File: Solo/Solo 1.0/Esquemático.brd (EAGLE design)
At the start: 51 x 57 mm, 13 parts, among them Q1 IRF540, Q2 IRF540, Q3 IRF540

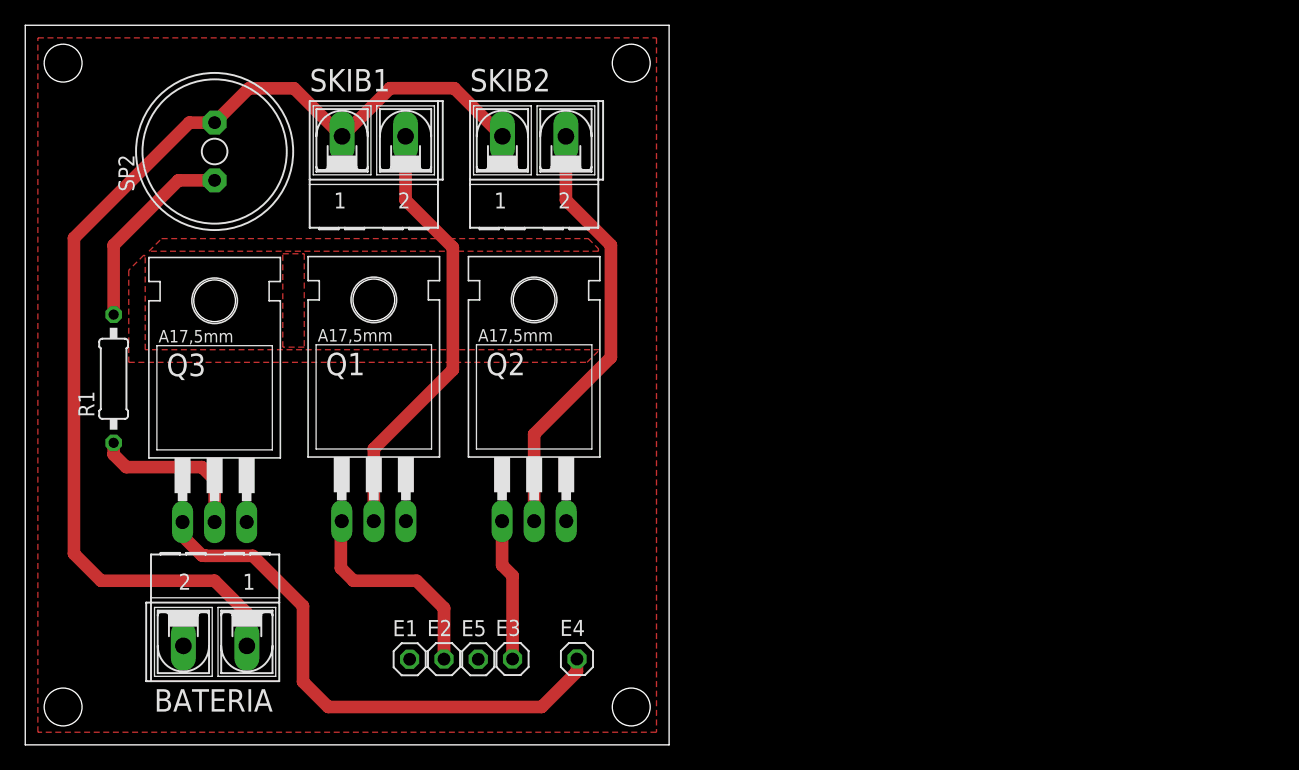
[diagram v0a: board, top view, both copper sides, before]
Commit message: Message
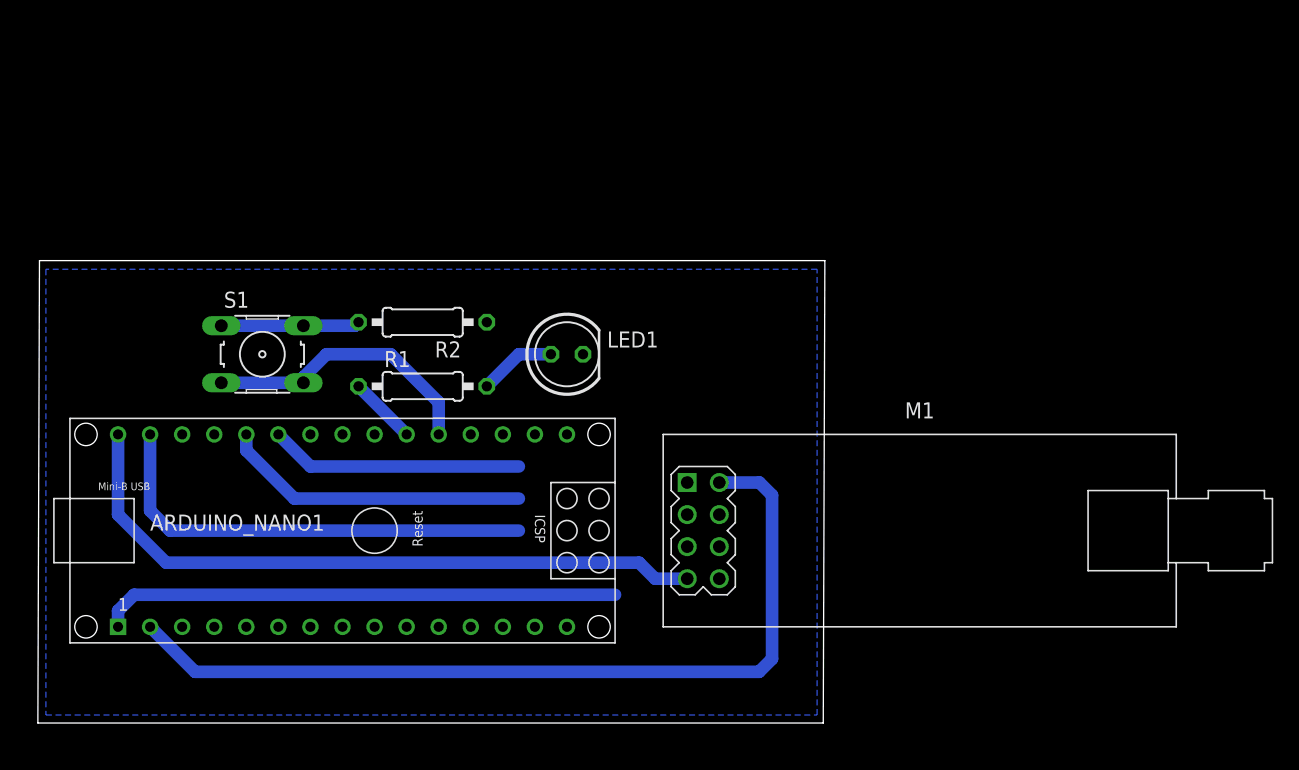
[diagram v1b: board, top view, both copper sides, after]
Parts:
- removed BATERIA, SKIB1, SKIB2: (no value), con-ptr500:AK500/2-H
- removed E1: 3V3, pinhead:1X01
- removed E2: SKIB1, pinhead:1X01
- removed E3: SKIB2, pinhead:1X01
- removed E4: BUZZER, pinhead:1X01
- removed E5: GND, pinhead:1X01
- removed Q1, Q2, Q3: IRF540, transistor-fet:TO220
- removed SP2: AL11P, buzzer:AL11P
- added ARDUINO_NANO1: (no value), ArduinoNanoV30:ARDUINO_NANO
- added LED1: (no value), led:LED5MM
- added M1: WIRELESS-NRF24L01-PA-EXT, modules:WIRELESS-NRF24L01-PA-EXT
- added R2: (no value), rcl:0207/10
- added S1: (no value), switch-omron:B3F-10XX
- R1: value 330 -> (none)
- moved R1 24.5 mm to (30.5, 25.4), turned to 0 degrees
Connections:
- removed net 3.3V: E1.1
- removed net BUZZER: E4.1, Q3.1
- removed net S1: Q1.2, SKIB1.2
- removed net S2: Q2.2, SKIB2.2
- removed net SKIB1: E2.1, Q1.1
- removed net SKIB2: E3.1, Q2.1
- removed net VCC: BATERIA.1, SKIB1.1, SKIB2.1, SP2.+
- new net 5V: ARDUINO_NANO1.12
- new net N$1: LED1.A, R1.2
- new net N$10: ARDUINO_NANO1.2, M1.2
- new net N$3: R2.2, S1.1, S1.2
- new net N$5: ARDUINO_NANO1.1, M1.5
- new net N$6: ARDUINO_NANO1.30, M1.7
- new net N$7: ARDUINO_NANO1.29, M1.6
- new net N$8: ARDUINO_NANO1.25, M1.3
- new net N$9: ARDUINO_NANO1.26, M1.4
- new net VIN: ARDUINO_NANO1.15
- net GND: now also ARDUINO_NANO1.14, ARDUINO_NANO1.19, LED1.K, M1.1, R2.1; no longer BATERIA.2, E5.1, Q1.3, Q2.3, Q3.3
- net N$2: now also ARDUINO_NANO1.20, S1.3, S1.4; no longer Q3.2, R1.1
- net N$4: now also ARDUINO_NANO1.21, R1.1; no longer R1.2, SP2.-
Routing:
- net VCC: track 86.8 -> 0.00 mm
- net N$10: track 0.00 -> 68.7 mm
- net N$6: track 0.00 -> 53.5 mm
- net BUZZER: track 43.6 -> 0.00 mm
- net N$5: track 0.00 -> 41.2 mm
- net N$7: track 0.00 -> 35.9 mm
- net S1: track 34.6 -> 0.00 mm
- net S2: track 34.5 -> 0.00 mm
- net N$9: track 0.00 -> 24.4 mm
- net N$8: track 0.00 -> 20.1 mm
- net SKIB1: track 17.3 -> 0.00 mm
- net SKIB2: track 11.3 -> 0.00 mm
- net N$3: track 0.00 -> 11.0 mm
- net N$4: track 15.6 -> 5.39 mm
- net N$2: track 13.1 -> 22.7 mm
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- added copper zone on layer 16, net GND
- removed copper zone on layer 1, net DS
- removed copper zone on layer 1, net GND
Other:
- board size 51 x 57 mm -> 62.3 x 36.6 mm

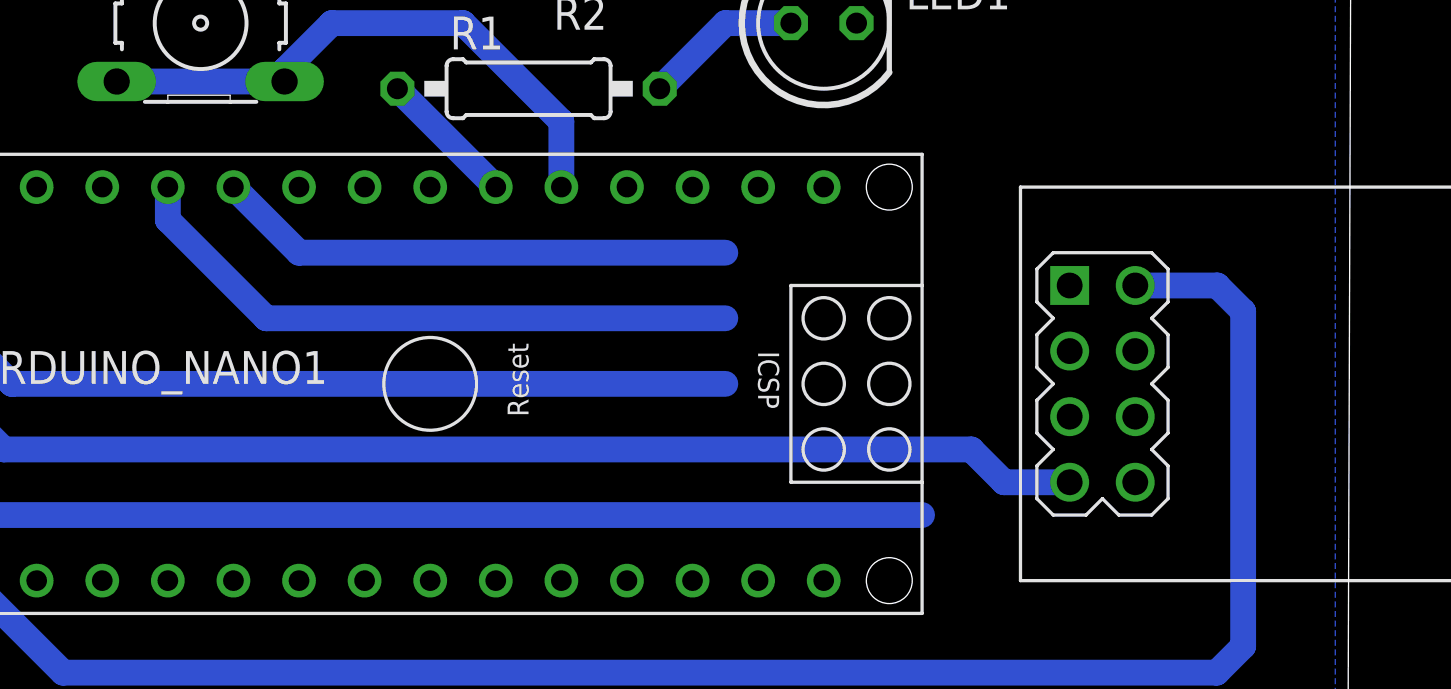
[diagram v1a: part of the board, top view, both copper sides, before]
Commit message: Upgrage
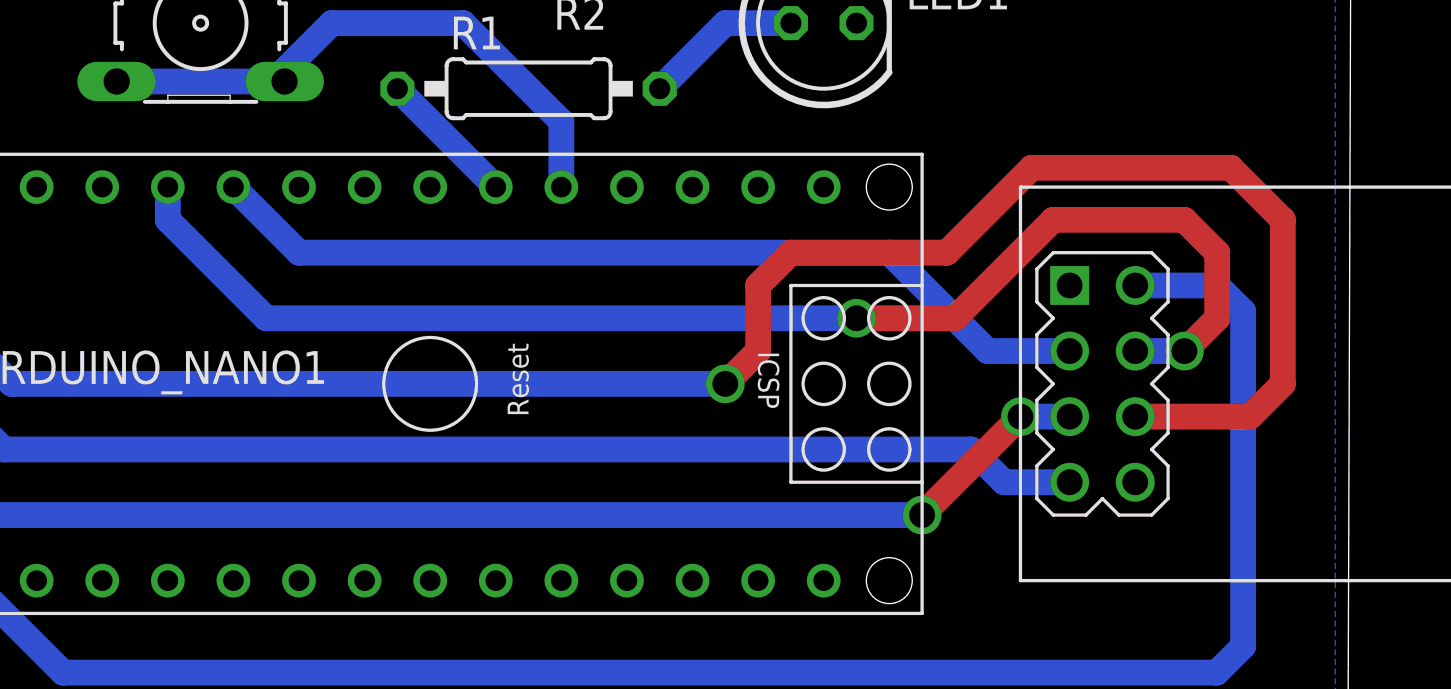
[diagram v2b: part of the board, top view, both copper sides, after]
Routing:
- net N$7: track 35.9 -> 75.9 mm, vias 0 -> 1
- net N$9: track 24.4 -> 51.8 mm, vias 0 -> 2
- net N$8: track 20.1 -> 35.0 mm
- net N$5: track 41.2 -> 48.5 mm, vias 0 -> 2
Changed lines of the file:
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@@
 <wire x1="6.35" y1="6.35" x2="6.35" y2="7.62" width="1" layer="16"/>
 <wire x1="6.35" y1="7.62" x2="7.62" y2="8.89" width="1" layer="16"/>
+<via x="45.72" y="8.89" extent="1-16" drill="1"/>
+<wire x1="49.53" y1="12.7" x2="45.72" y2="8.89" width="1" layer="1"/>
+<via x="49.53" y="12.7" extent="1-16" drill="1"/>
+<wire x1="49.53" y1="12.7" x2="51.435" y2="12.7" width="1" layer="16"/>
 <wire x1="7.62" y1="8.89" x2="45.72" y2="8.89" width="1" layer="16"/>
-<wire x1="45.72" y1="8.89" x2="51.435" y2="12.7" width="0" layer="19" extent="16-16"/>
 </signal>
 <signal name="N$6">
@@
 <wire x1="8.89" y1="15.55105625" x2="10.47105625" y2="13.97" width="1" layer="16"/>
 <wire x1="10.47105625" y1="13.97" x2="38.1" y2="13.97" width="1" layer="16"/>
-<wire x1="38.1" y1="13.97" x2="53.975" y2="12.7" width="0" layer="19" extent="16-16"/>
+<via x="38.1" y="13.97" extent="1-16" drill="1"/>
+<wire x1="38.1" y1="13.97" x2="39.37" y2="15.24" width="1" layer="1"/>
+<wire x1="39.37" y1="17.78" x2="40.64" y2="19.05" width="1" layer="1"/>
+<wire x1="40.64" y1="19.05" x2="46.67894375" y2="19.05" width="1" layer="1"/>
+<wire x1="57.674" y1="22.336" x2="59.69" y2="20.32" width="1" layer="1"/>
+<wire x1="59.69" y1="20.32" x2="59.69" y2="13.97" width="1" layer="1"/>
+<wire x1="59.69" y1="13.97" x2="58.42" y2="12.7" width="1" layer="1"/>
+<wire x1="58.42" y1="12.7" x2="53.975" y2="12.7" width="1" layer="1"/>
+<wire x1="39.37" y1="15.24" x2="39.37" y2="17.78" width="1" layer="1"/>
+<wire x1="46.67894375" y1="19.05" x2="49.96494375" y2="22.336" width="1" layer="1"/>
+<wire x1="49.96494375" y1="22.336" x2="57.674" y2="22.336" width="1" layer="1"/>
 </signal>
 <signal name="N$8">
@@
 <contactref element="ARDUINO_NANO1" pad="25"/>
 <wire x1="19.05" y1="21.59" x2="21.59" y2="19.05" width="1" layer="16"/>
-<wire x1="21.59" y1="19.05" x2="38.1" y2="19.05" width="1" layer="16"/>
-<wire x1="38.1" y1="19.05" x2="51.435" y2="15.24" width="0" layer="19" extent="16-16"/>
+<wire x1="44.45" y1="19.05" x2="48.26" y2="15.24" width="1" layer="16"/>
+<wire x1="48.26" y1="15.24" x2="51.435" y2="15.24" width="1" layer="16"/>
+<wire x1="21.59" y1="19.05" x2="44.45" y2="19.05" width="1" layer="16"/>
 </signal>
 <signal name="N$9">
 <contactref element="ARDUINO_NANO1" pad="26"/>
 <contactref element="M1" pad="4"/>
-<wire x1="20.32" y1="16.51" x2="16.51" y2="20.32" width="1" layer="16"/>
+<wire x1="16.51" y1="20.32" x2="20.32" y2="16.51" width="1" layer="16"/>
 <wire x1="16.51" y1="21.59" x2="16.51" y2="20.32" width="1" layer="16"/>
-<wire x1="20.32" y1="16.51" x2="38.1" y2="16.51" width="1" layer="16"/>
-<wire x1="38.1" y1="16.51" x2="53.975" y2="15.24" width="0" layer="19" extent="16-16"/>
+<via x="43.18" y="16.51" extent="1-16" drill="1"/>
+<wire x1="50.8" y1="20.32" x2="46.99" y2="16.51" width="1" layer="1"/>
+<wire x1="43.18" y1="16.51" x2="46.99" y2="16.51" width="1" layer="1"/>
+<wire x1="57.15" y1="19.05" x2="57.15" y2="16.51" width="1" layer="1"/>
+<via x="55.88" y="15.24" extent="1-16" drill="1"/>
+<wire x1="55.88" y1="15.24" x2="53.975" y2="15.24" width="1" layer="16"/>
+<wire x1="20.32" y1="16.51" x2="43.18" y2="16.51" width="1" layer="16"/>
+<wire x1="50.8" y1="20.32" x2="55.88" y2="20.32" width="1" layer="1"/>
+<wire x1="55.88" y1="20.32" x2="57.15" y2="19.05" width="1" layer="1"/>
+<wire x1="57.15" y1="16.51" x2="55.88" y2="15.24" width="1" layer="1"/>
 </signal>
 <signal name="N$10">
-<contactref element="M1" pad="2"/>
 <contactref element="ARDUINO_NANO1" pad="2"/>
 <wire x1="8.89" y1="6.35" x2="12.454" y2="2.786" width="1" layer="16"/>
 <wire x1="57.13" y1="2.786" x2="58.154" y2="3.81" width="1" layer="16"/>
 <wire x1="58.154" y1="16.776" x2="57.15" y2="17.78" width="1" layer="16"/>
-<wire x1="57.15" y1="17.78" x2="53.975" y2="17.78" width="1" layer="16"/>
 <wire x1="12.454" y1="2.786" x2="57.13" y2="2.786" width="1" layer="16"/>
 <wire x1="58.154" y1="3.81" x2="58.154" y2="16.776" width="1" layer="16"/>
+<contactref element="M1" pad="2"/>
+<wire x1="57.15" y1="17.78" x2="53.975" y2="17.78" width="1" layer="16"/>
 </signal>
 </signals>
@@
 <mfgpreviewcolor name="substratecolor" color="0xFF786E46"/>
 </mfgpreviewcolors>
+<errors>
+</errors>
 </board>
 </drawing>
